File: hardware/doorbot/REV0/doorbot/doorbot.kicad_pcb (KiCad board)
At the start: 2 copper layers, 39 parts, among them J1 Raspberry_Pi_2_3, J2 Screw_Terminal_01x12, J3 PoE Passthrough, Q1 2N7002, U1 ATmega328P-AU, U2 TLP291, U3 TLP291, U4 TLP291, U5 TLP291, U6 TLP291, U7 DRV103, U8 MC78L05_SOT89

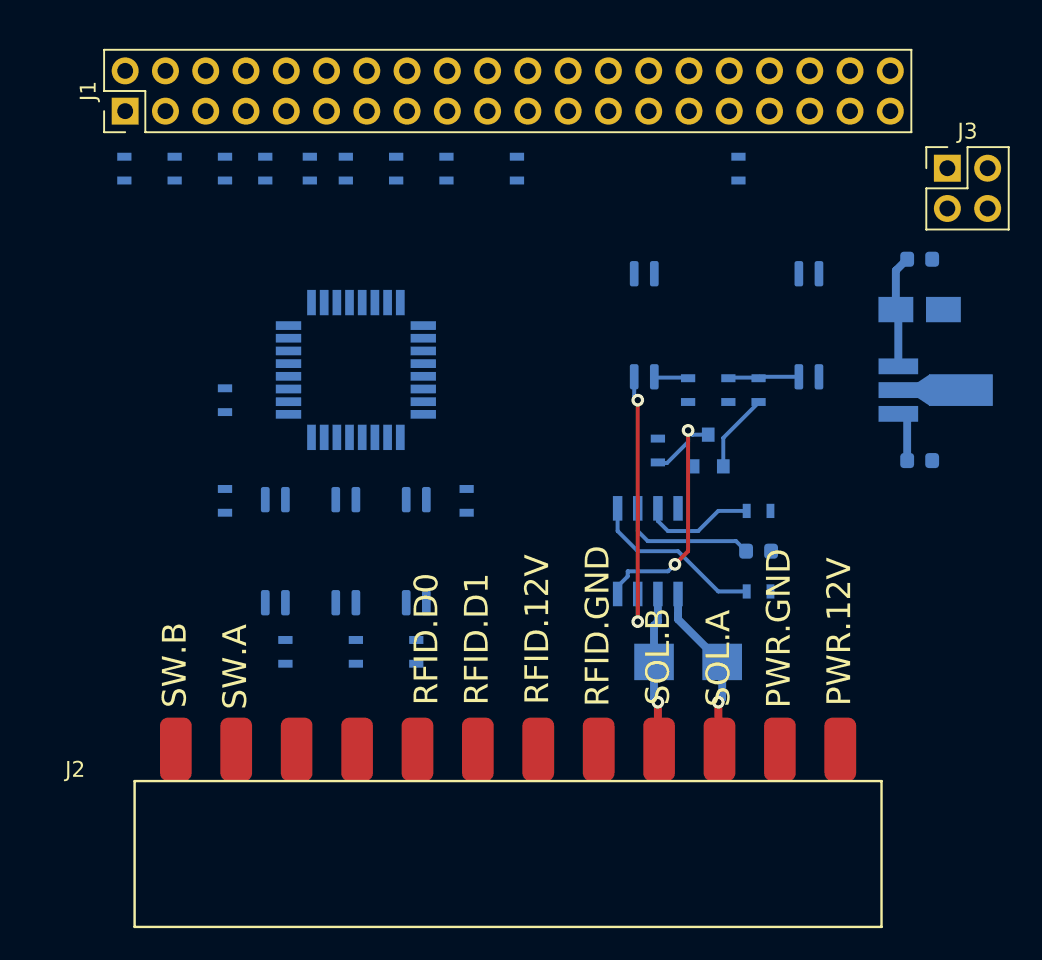
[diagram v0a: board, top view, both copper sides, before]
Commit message: moar doorbot pcb
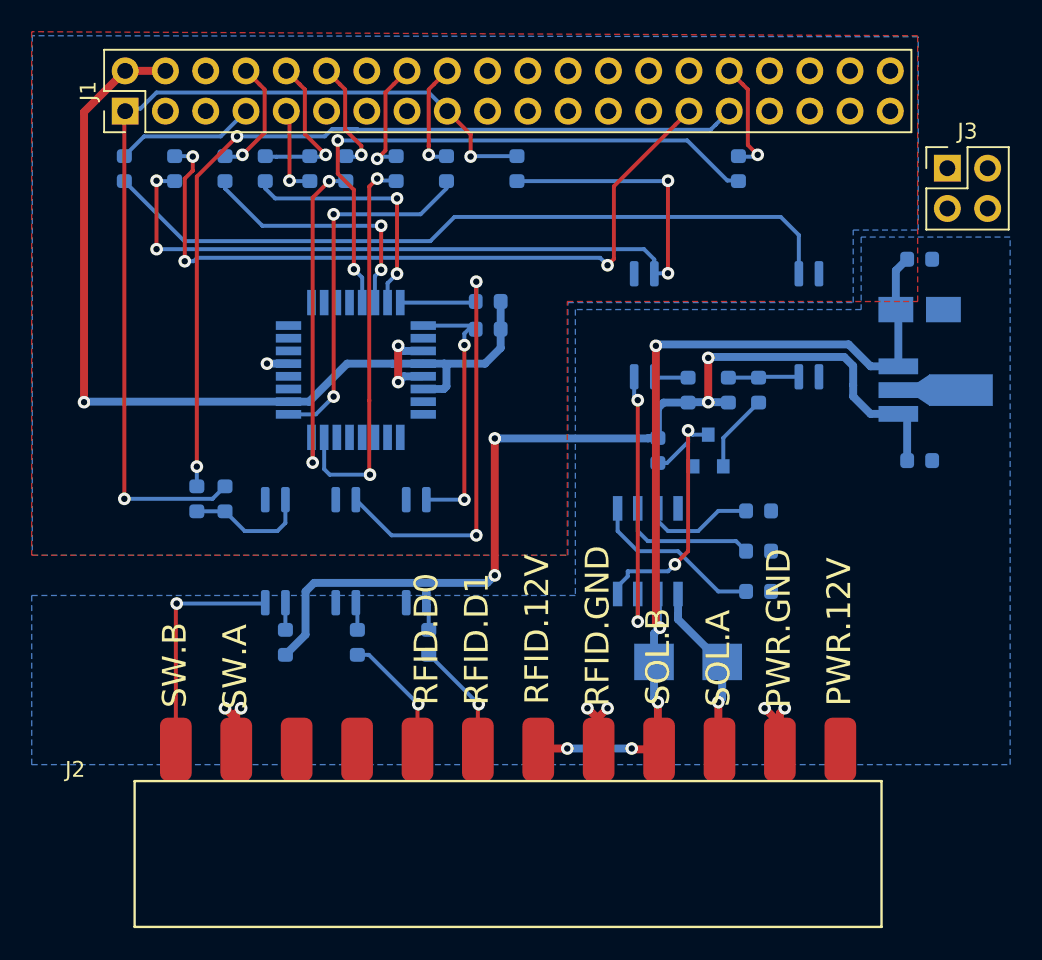
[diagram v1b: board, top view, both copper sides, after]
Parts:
- added R23: 47, Resistor_SMD:R_0603_1608Metric, B.Cu at (118.9, 91.9)
- R1, R10, R11, R12, R13, R14, R15, R16, R17, R18, R19, R2, R20, R21, R22, R3, R4, R5, R6, R7, R8, R9: footprint Resistors_SMD:R_0603 -> Resistor_SMD:R_0603_1608Metric
- moved R11 17.7 mm to (137.2, 79.5), turned to 180 degrees
- moved R12 10.9 mm to (137.2, 81.2), turned to 180 degrees
- moved R17 0.99 mm to (133.5, 101.0)
- moved R16 0.61 mm to (129.0, 101.0)
- moved R18 0.60 mm to (124.5, 101.0)
- moved R10 0.13 mm to (120.7, 91.9)
- turned R19 to 270 degrees
- turned R20 to 270 degrees
- turned R21 to 270 degrees
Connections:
- R4 pad 2: Net-(J1-Pad5) -> Net-(J1-Pad29)
- R6 pad 2: Net-(J1-Pad3) -> Net-(J1-Pad7)
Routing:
- net +5VA: track 3.35 -> 63.1 mm, vias 0 -> 4
- net +3V3: track 0.00 -> 58.9 mm, vias 0 -> 2
- net +5V: track 0.00 -> 58.2 mm, vias 0 -> 1
- net Net-(J1-Pad31): track 0.00 -> 54.9 mm, vias 0 -> 2
- net Net-(R4-Pad1): track 0.00 -> 54.3 mm, vias 0 -> 4
- net Net-(R6-Pad1): track 0.00 -> 47.7 mm
- net Net-(J1-Pad29): track 0.00 -> 46.8 mm, vias 0 -> 3
- net +12VA: track 17.1 -> 58.7 mm, vias 1 -> 5
- net /AT_RST: track 0.00 -> 37.2 mm, vias 0 -> 2
- net /WG_D0: track 0.00 -> 30.6 mm, vias 0 -> 2
- net /AT_MOSI: track 0.00 -> 25.2 mm, vias 0 -> 2
- net /AT_SCK: track 0.00 -> 23.1 mm, vias 0 -> 2
- net /AT_MISO: track 0.00 -> 20.9 mm, vias 0 -> 2
- net Earth: track 0.00 -> 17.0 mm, vias 0 -> 6
- net /WG_D1: track 0.00 -> 17.0 mm, vias 0 -> 2
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- added copper zone on B.Cu, net Earth
- added copper zone on B.Cu, net GND
- added copper zone on F.Cu, net GND
